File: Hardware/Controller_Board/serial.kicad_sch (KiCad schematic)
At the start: 29 parts, among them U201 XC7A35T-CPG236, U501 FT232H, U502 93LC56B, Y501 12MHz

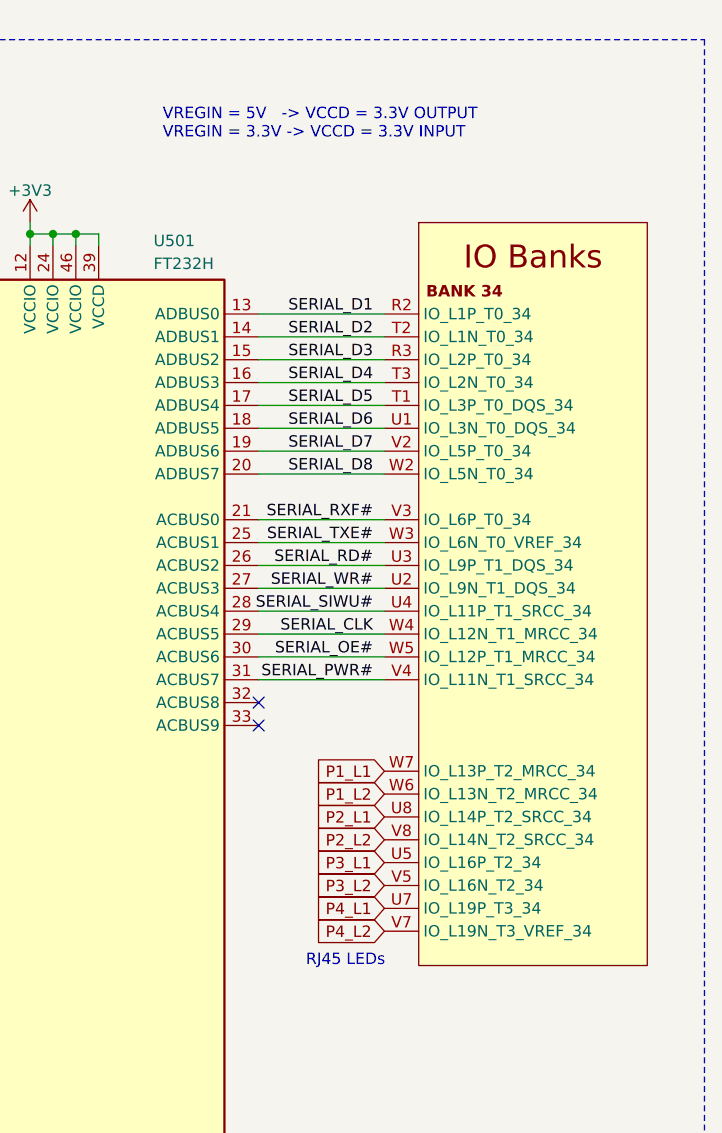
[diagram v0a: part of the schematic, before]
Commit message: Commit before upgrading to KiCad 10.0
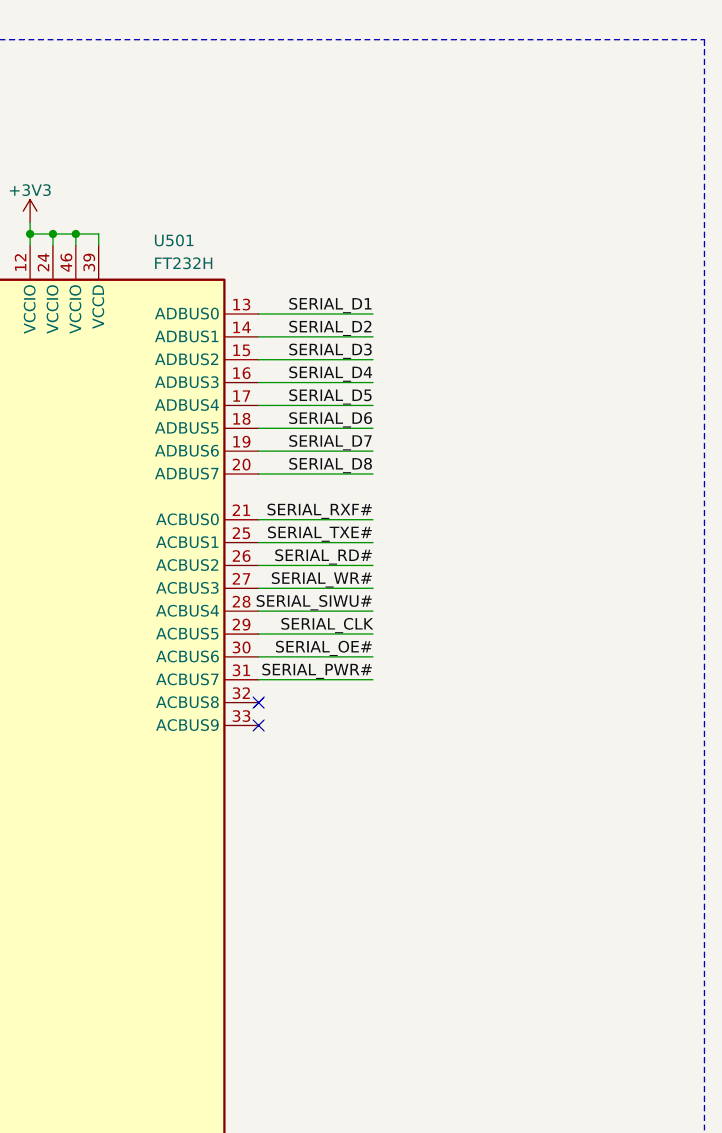
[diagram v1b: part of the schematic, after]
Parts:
- removed U201: XC7A35T-CPG236, Package_BGA:Xilinx_CPG236, symbol Custom_VoxLink_Symbols:XC7A35T-CPG236
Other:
- note removed: "RJ45 LEDs"
- note removed: "VREGIN = 5V -> VCCD = 3.3V OUTPUT VREGIN = 3.3V -> VCCD = 3.3V INPUT"
